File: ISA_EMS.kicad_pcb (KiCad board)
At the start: 2 copper layers, 176.5 x 85.1 mm, 49 parts, among them J1 ISA BUS, J2 EMS Address, U10 74HCT32, U11 74HCT04, U12 74LS245, U13 AS6C4008-55PCN, U14 AS6C4008-55PCN, U15 AS6C4008-55PCN, U16 AS6C4008-55PCN, U17 74HCT138, U18 74HCT573, U19 74HCT573, U20 74HCT573, U21 74HCT573, U3 AS6C4008-55PCN, U4 AS6C4008-55PCN, U5 AS6C4008-55PCN, U6 AS6C4008-55PCN, U7 74HCT688, U8 74HCT688, U9 74HCT139

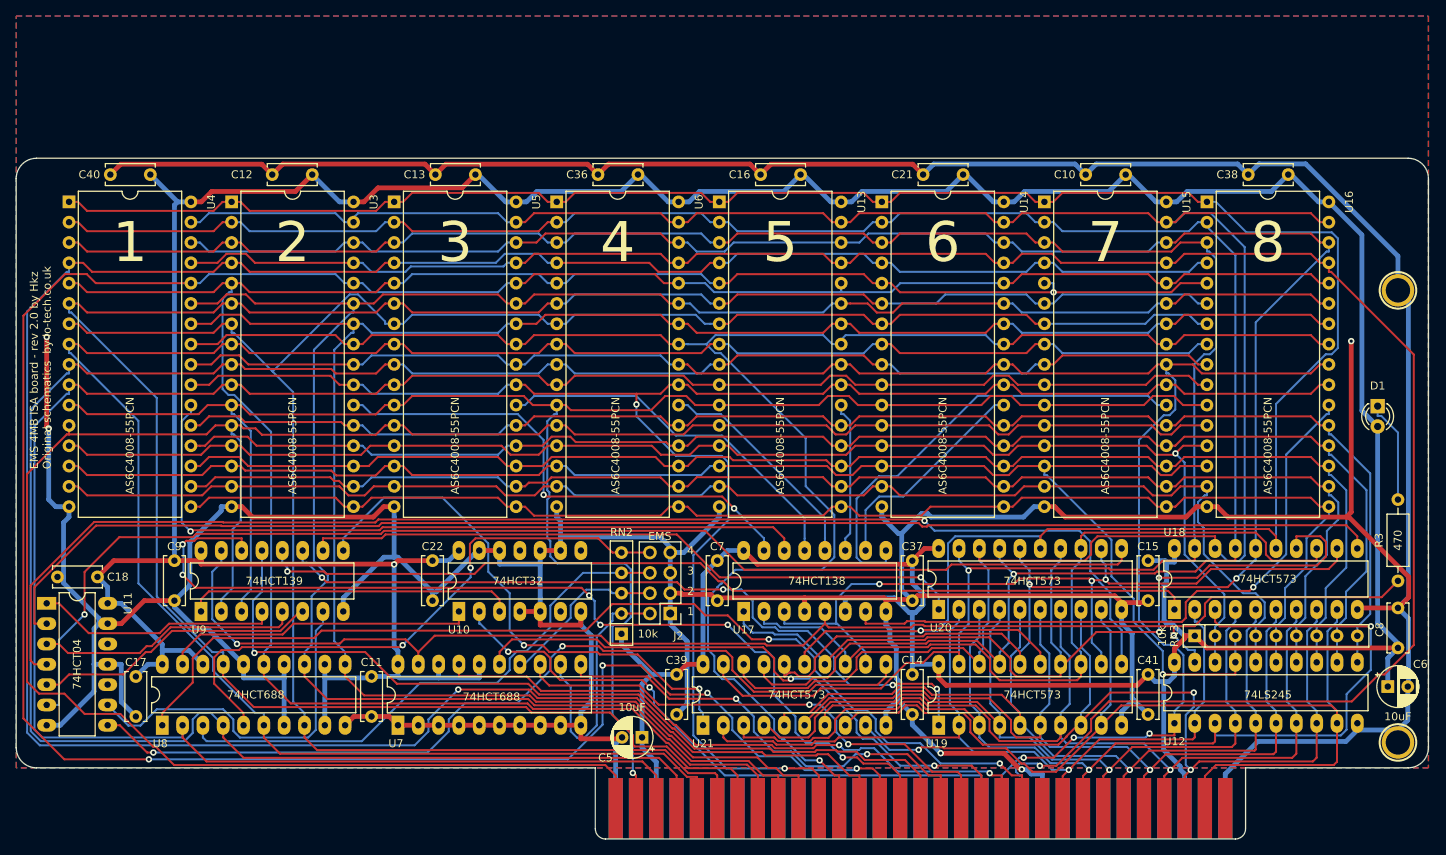
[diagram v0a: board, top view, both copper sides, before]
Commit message: Initial import to KiCad 7
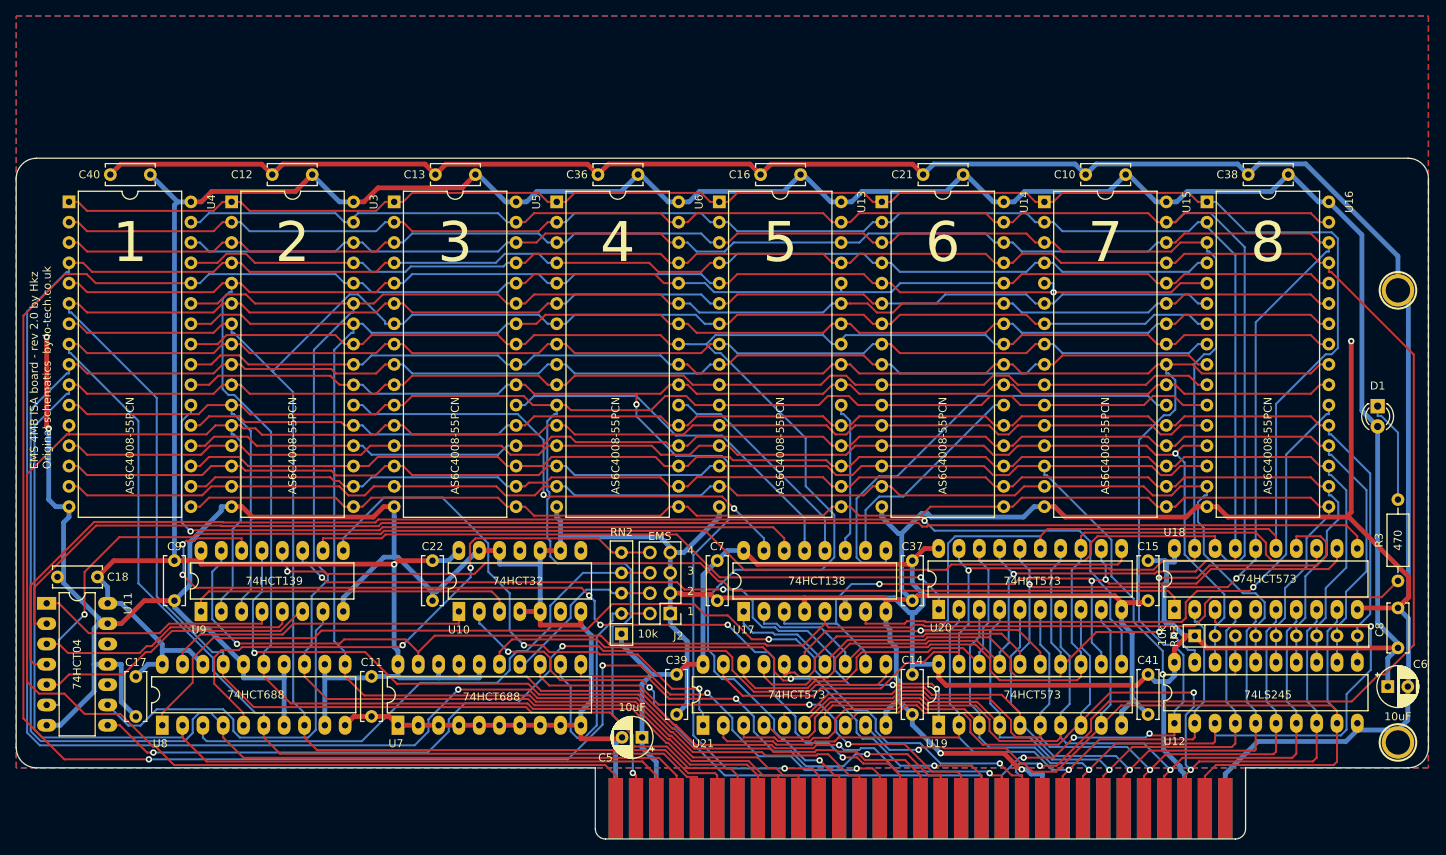
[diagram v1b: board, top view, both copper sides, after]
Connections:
- net /~IOW renamed /~{IOW}
- net /~MEMR renamed /~{MEMR}
- net /~MEMW renamed /~{MEMW}
- net /~RAM-CS0 renamed /~{RAM-CS0}
- net /~RAM-CS1 renamed /~{RAM-CS1}
- net /~RAM-CS2 renamed /~{RAM-CS2}
- net /~RAM-CS3 renamed /~{RAM-CS3}
- net /~RAM-CS4 renamed /~{RAM-CS4}
- net /~RAM-CS5 renamed /~{RAM-CS5}
- net /~RAM-CS6 renamed /~{RAM-CS6}
- net /~RAM-CS7 renamed /~{RAM-CS7}
- net /~RAM-SELECT renamed /~{RAM-SELECT}
- net /~REG0-OE renamed /~{REG0-OE}
- net /~REG1-OE renamed /~{REG1-OE}
- net /~REG2-OE renamed /~{REG2-OE}
- net /~REG3-OE renamed /~{REG3-OE}
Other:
- net class Default removed
- net class POWER removed
- net class POWR_SMALL removed
